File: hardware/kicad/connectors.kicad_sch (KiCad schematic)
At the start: 10 parts, among them J701 RC receiver, J702 GPS, J703 Aux I2C, J704 Buzzer, J705 LED strip, Q701 AO3400A

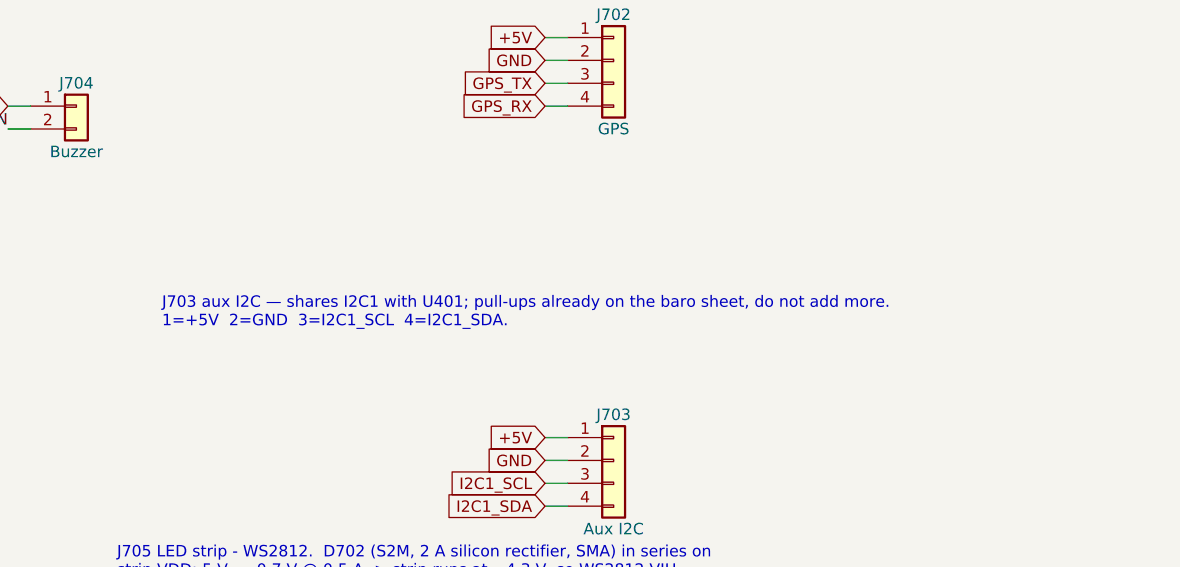
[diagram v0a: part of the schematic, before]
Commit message: Review fixes: series protection R, I2C1 2.2k, C102 50V, gate & buck soft-start
7.f - PA2/PA3 = TTa (not 5V tolerant), PD2 = FT (5V tolerant) per STM32F405
DS8626. Add series R on the STM32 pin side: R205 1k ESC_TLM, R206 1k GPS_TX,
R207 1k GPS_RX (limits fault injection into PA2/PA3 to ~1.2 mA on a 5V UART).

3.a - Cross-domain series R: R208 470 BRIDGE_TX, R209 470 BRIDGE_RX, R210 470
ESP_STM_NRST (R203 pull-down + Q201 gate kept on the local node -> ESP-absent
fail-safe preserved).

6.a - I2C1 pull-ups R401/R402 4.7k -> 2.2k (C4190). With J703 cabled
(~90-100 pF): t_r ~= 186 ns < 300 ns (400 kHz); sink 1.4 mA at VOL.

1.a - C102 10uF 25V -> 50V (C138687), for 4S input transients + DC-bias
derating.

7.a - Inrush handled by a BUILD REQUIREMENT: anti-spark XT60/XT90 on the
battery lead (a single reverse-polarity P-FET cannot soft-start plug-in
inrush - body diode is forward). C114 100nF gate-source stays for a
controlled ~7 ms gate turn-on / softer VBAT_SW rise. J101 annotated.

MP2307 SS: C115 100nF on the SS pin (was left open). t_ss ~= 15 ms per r1.9
-> +5V ramps 0->5 V charging C105+C113 (~46 uF) at ~15 mA, not the ~4 A
current limit. Project symbol MP2307DN pin 8 corrected NC -> SS (passive).

ERC: 0 errors / 0 isolated_pin_label / 2 known pin_to_pin warnings.

Co-Authored-By: Claude Sonnet 5 <noreply@anthropic.com>
Claude-Session: https://claude.ai/code/session_0171uwNh8K8uwZuWio9f35u1
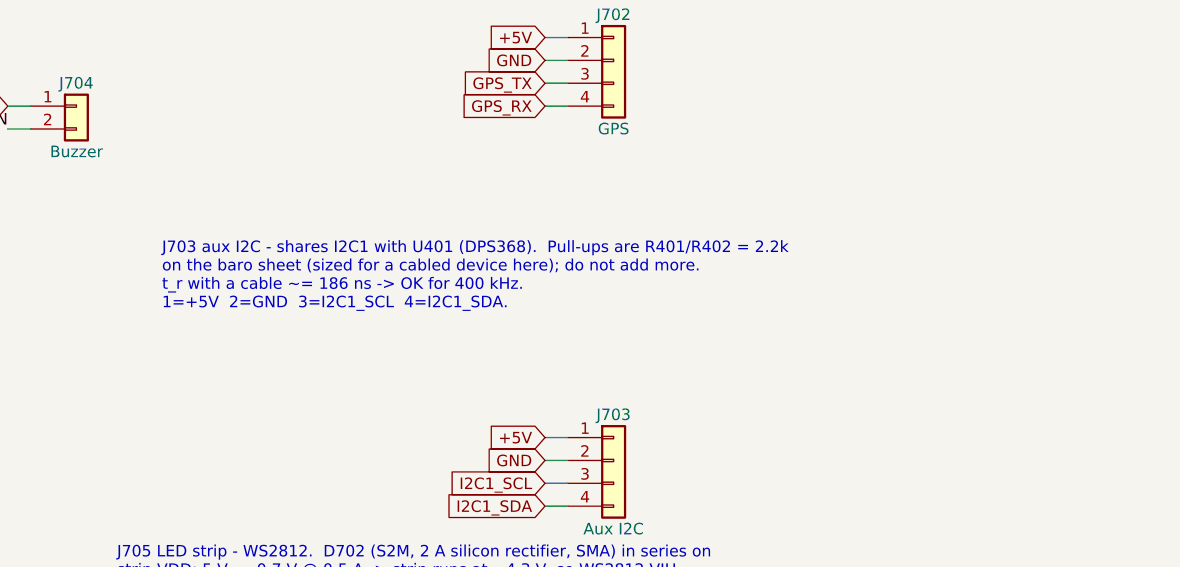
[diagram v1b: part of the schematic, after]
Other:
- note added: "J703 aux I2C - shares I2C1 with U401 (DPS368). Pull-ups are R401/R402 = 2.2k on the baro sheet (sized for a cabled device here); do not add more. t_r with a cable ~= 186 ns -> OK for 400 kHz. 1=+5V 2=GND 3=I2C1_SCL 4=I2C1_SDA."
- note removed: "J703 aux I2C — shares I2C1 with U401; pull-ups already on the baro sheet, do not add more. 1=+5V 2=GND 3=I2C1_SCL 4=I2C1_SDA."
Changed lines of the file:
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@@
-		)
-	)
-	(text "J703 aux I2C — shares I2C1 with U401; pull-ups already on the baro sheet, do not add more.\n1=+5V  2=GND  3=I2C1_SCL  4=I2C1_SDA."
-		(at 120 120 0)
-		(effects
-			(font
-				(size 1.27 1.27)
-			)
-			(justify left bottom)
 		)
 	)
@@
     (effects (font (size 1.27 1.27)) (justify left bottom))
   )
+  (text "J703 aux I2C - shares I2C1 with U401 (DPS368).  Pull-ups are R401/R402 = 2.2k\non the baro sheet (sized for a cabled device here); do not add more.\nt_r with a cable ~= 186 ns -> OK for 400 kHz.\n1=+5V  2=GND  3=I2C1_SCL  4=I2C1_SDA."
+    (at 120 118 0)
+    (effects (font (size 1.27 1.27)) (justify left bottom))
+  )
